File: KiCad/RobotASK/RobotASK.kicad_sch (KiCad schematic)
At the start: 14 parts, among them J1 Conn_01x04_Pin, J2 Conn_01x04_Pin, J3 Conn_01x04_Pin, J4 Conn_01x04_Pin, J5 Conn_01x04_Pin, J6 Conn_01x04_Pin, J7 Conn_01x02_Pin, J8 Conn_01x03_Pin, SW2 SW_Omron_B3FS, U1 ATmega328-P, Y1 16MHz

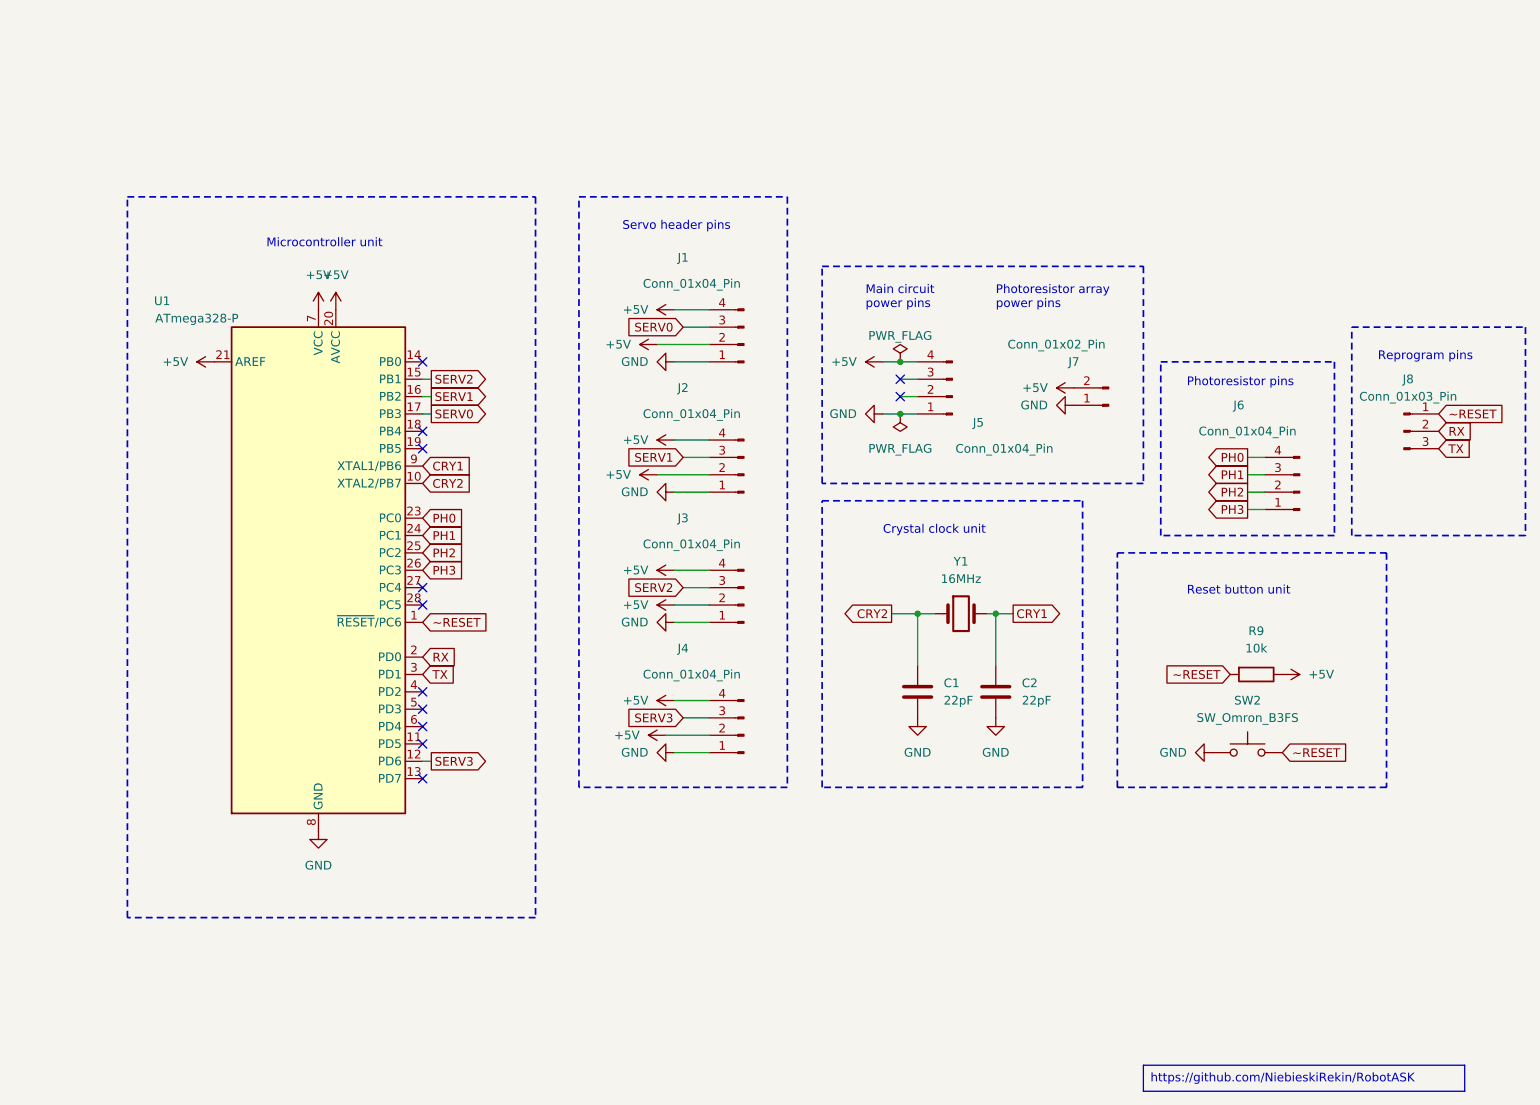
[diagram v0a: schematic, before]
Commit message: renders
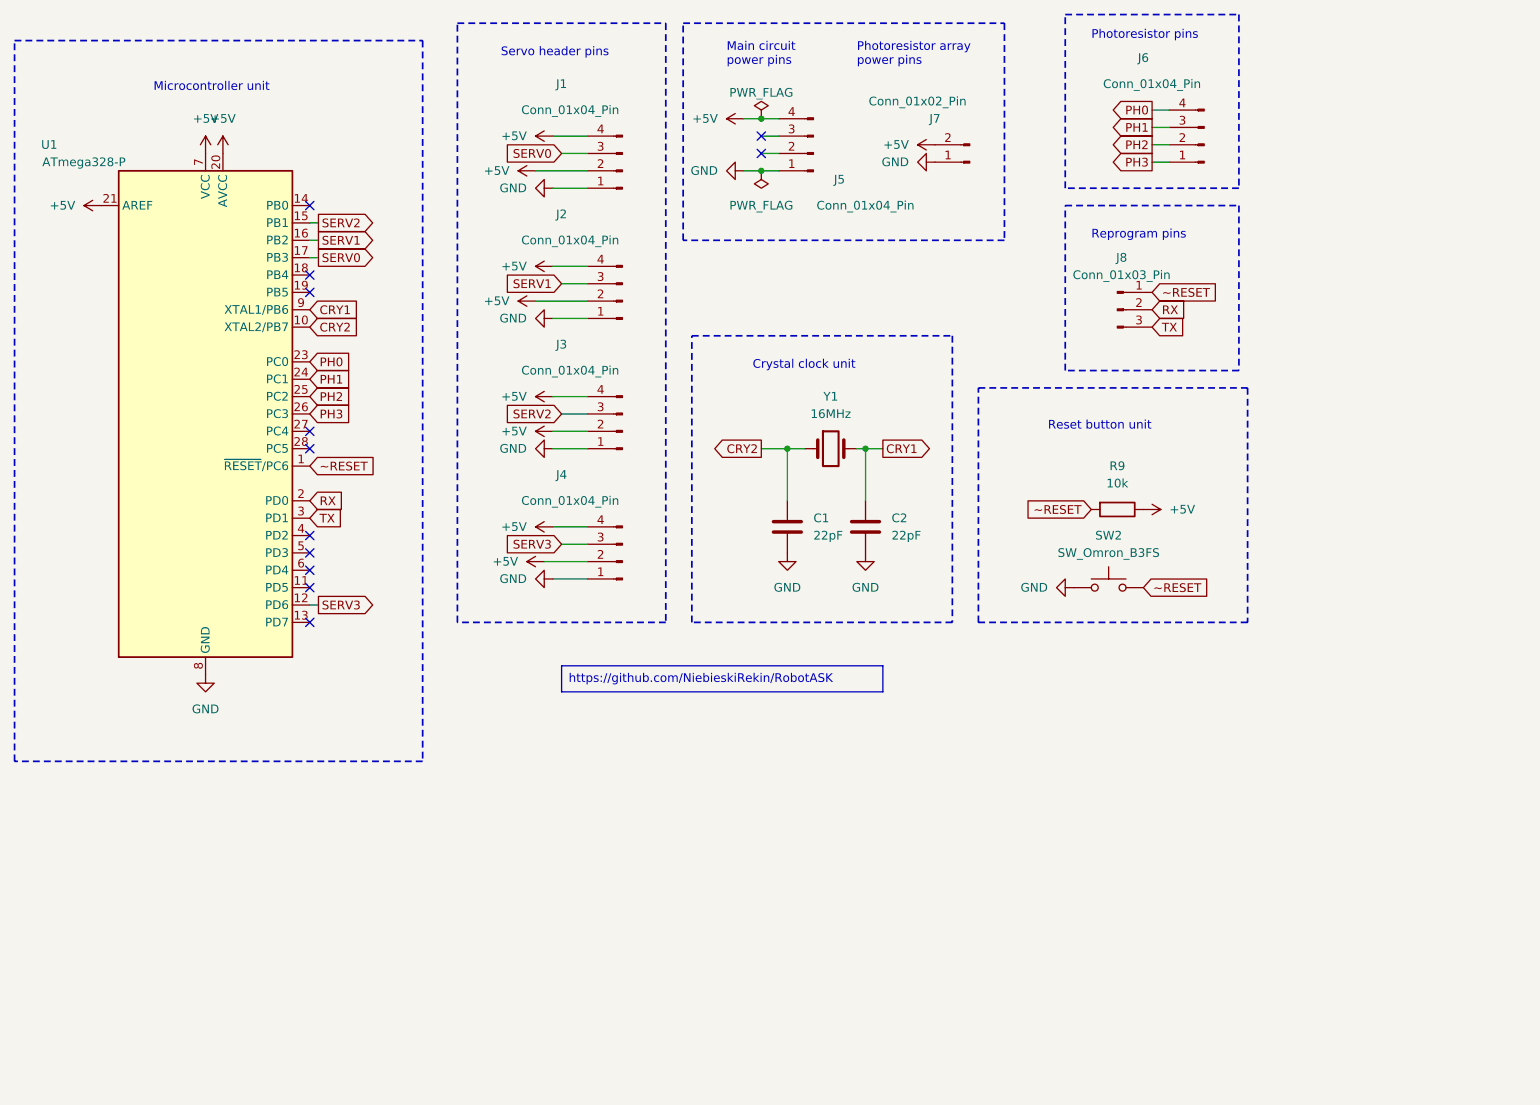
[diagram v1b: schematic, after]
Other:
- moved on the sheet: C1, C2, J1, J2, J3, J4, J5, J6, J7, J8, R9, SW2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
